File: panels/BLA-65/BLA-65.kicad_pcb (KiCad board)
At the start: 2 copper layers, 60.1 x 128.4 mm, 6 parts

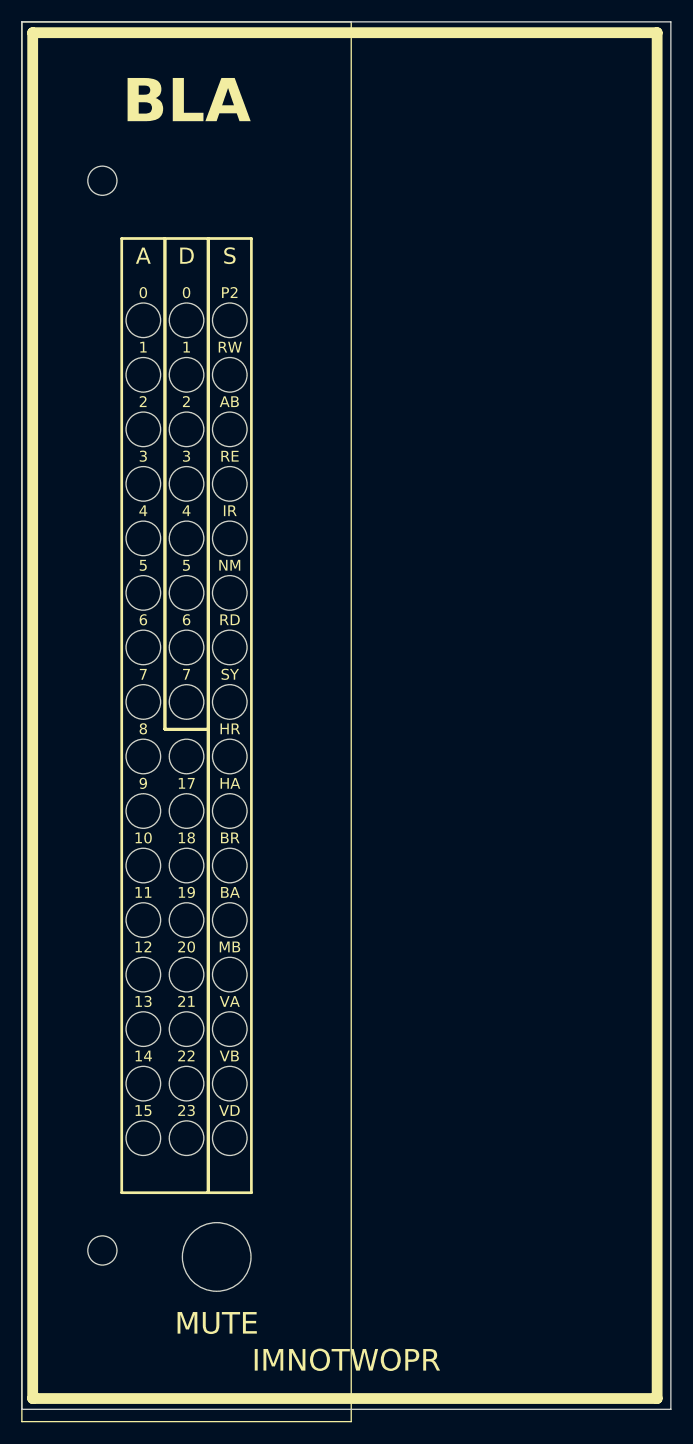
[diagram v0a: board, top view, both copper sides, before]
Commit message: bla panel
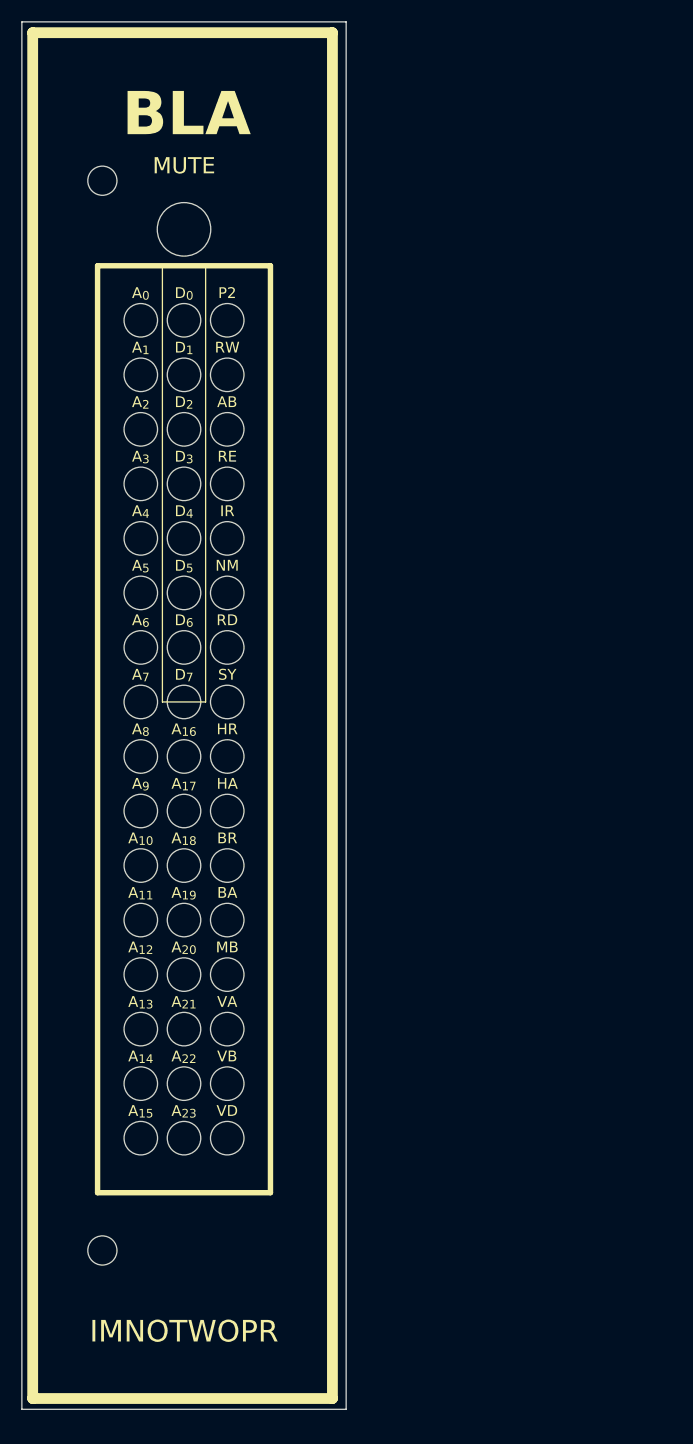
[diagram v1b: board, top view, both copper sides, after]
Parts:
- removed H2: TOP RIGHT, FormantKO-Panel:PanelMountingHole
- removed H4: BOTTOM RIGHT, FormantKO-Panel:PanelMountingHole
- removed the REF** at (84.3, 153.8)
- added REF**: Panel_LED_3.0mm, IMNOTWOPR:Panel_LED_3.0mm, F.Cu at (85.3, 92.4)
- added REF**: Panel_LED_3.0mm, IMNOTWOPR:Panel_LED_3.0mm, F.Cu at (85.3, 137.8)
- added REF**: Panel_LED_3.0mm, IMNOTWOPR:Panel_LED_3.0mm, F.Cu at (77.3, 92.4)
- added REF**: Panel_LED_3.0mm, IMNOTWOPR:Panel_LED_3.0mm, F.Cu at (81.3, 132.7)
- added REF**: Panel_LED_3.0mm, IMNOTWOPR:Panel_LED_3.0mm, F.Cu at (81.3, 72.2)
- added REF**: Panel_LED_3.0mm, IMNOTWOPR:Panel_LED_3.0mm, F.Cu at (85.3, 77.2)
- added REF**: Panel_LED_3.0mm, IMNOTWOPR:Panel_LED_3.0mm, F.Cu at (81.3, 117.6)
- added REF**: Panel_LED_3.0mm, IMNOTWOPR:Panel_LED_3.0mm, F.Cu at (77.3, 132.7)
- added REF**: Panel_LED_3.0mm, IMNOTWOPR:Panel_LED_3.0mm, F.Cu at (81.3, 137.8)
- added REF**: Panel_LED_3.0mm, IMNOTWOPR:Panel_LED_3.0mm, F.Cu at (85.3, 107.5)
- added REF**: Panel_LED_3.0mm, IMNOTWOPR:Panel_LED_3.0mm, F.Cu at (77.3, 102.5)
- added REF**: Panel_LED_3.0mm, IMNOTWOPR:Panel_LED_3.0mm, F.Cu at (81.3, 87.3)
- added REF**: Panel_LED_3.0mm, IMNOTWOPR:Panel_LED_3.0mm, F.Cu at (85.3, 122.6)
- added REF**: Panel_LED_3.0mm, IMNOTWOPR:Panel_LED_3.0mm, F.Cu at (77.3, 72.2)
- added REF**: Panel_LED_3.0mm, IMNOTWOPR:Panel_LED_3.0mm, F.Cu at (85.3, 127.7)
- added REF**: Panel_LED_3.0mm, IMNOTWOPR:Panel_LED_3.0mm, F.Cu at (77.3, 82.3)
- added REF**: Panel_LED_3.0mm, IMNOTWOPR:Panel_LED_3.0mm, F.Cu at (85.3, 132.7)
- added REF**: Panel_LED_3.0mm, IMNOTWOPR:Panel_LED_3.0mm, F.Cu at (77.3, 142.8)
- added REF**: Panel_LED_3.0mm, IMNOTWOPR:Panel_LED_3.0mm, F.Cu at (85.3, 87.3)
- added REF**: Panel_LED_3.0mm, IMNOTWOPR:Panel_LED_3.0mm, F.Cu at (85.3, 67.1)
- added REF**: Panel_LED_3.0mm, IMNOTWOPR:Panel_LED_3.0mm, F.Cu at (85.3, 142.8)
- added REF**: Panel_LED_3.0mm, IMNOTWOPR:Panel_LED_3.0mm, F.Cu at (85.3, 72.2)
- added REF**: Panel_LED_3.0mm, IMNOTWOPR:Panel_LED_3.0mm, F.Cu at (77.3, 77.2)
- added REF**: Panel_LED_3.0mm, IMNOTWOPR:Panel_LED_3.0mm, F.Cu at (81.3, 102.5)
- added REF**: Panel_LED_3.0mm, IMNOTWOPR:Panel_LED_3.0mm, F.Cu at (81.3, 82.3)
- added REF**: Panel_LED_3.0mm, IMNOTWOPR:Panel_LED_3.0mm, F.Cu at (81.3, 92.4)
- added REF**: Panel_LED_3.0mm, IMNOTWOPR:Panel_LED_3.0mm, F.Cu at (85.3, 117.6)
- added REF**: Panel_LED_3.0mm, IMNOTWOPR:Panel_LED_3.0mm, F.Cu at (77.3, 87.3)
- added REF**: Panel_LED_3.0mm, IMNOTWOPR:Panel_LED_3.0mm, F.Cu at (77.3, 67.1)
- added REF**: Panel_LED_3.0mm, IMNOTWOPR:Panel_LED_3.0mm, F.Cu at (85.3, 102.5)
- added REF**: Panel_LED_3.0mm, IMNOTWOPR:Panel_LED_3.0mm, F.Cu at (77.3, 97.4)
- added REF**: Panel_LED_3.0mm, IMNOTWOPR:Panel_LED_3.0mm, F.Cu at (81.3, 112.5)
- added REF**: Panel_LED_3.0mm, IMNOTWOPR:Panel_LED_3.0mm, F.Cu at (85.3, 97.4)
- added REF**: Panel_LED_3.0mm, IMNOTWOPR:Panel_LED_3.0mm, F.Cu at (77.3, 112.5)
- added REF**: Panel_LED_3.0mm, IMNOTWOPR:Panel_LED_3.0mm, F.Cu at (85.3, 82.3)
- added REF**: Panel_LED_3.0mm, IMNOTWOPR:Panel_LED_3.0mm, F.Cu at (77.3, 127.7)
- added REF**: Panel_LED_3.0mm, IMNOTWOPR:Panel_LED_3.0mm, F.Cu at (81.3, 142.8)
- added REF**: Panel_LED_3.0mm, IMNOTWOPR:Panel_LED_3.0mm, F.Cu at (85.3, 112.5)
- added REF**: Panel_LED_3.0mm, IMNOTWOPR:Panel_LED_3.0mm, F.Cu at (77.3, 117.6)
- added REF**: Panel_LED_3.0mm, IMNOTWOPR:Panel_LED_3.0mm, F.Cu at (77.3, 122.6)
- added REF**: Panel_LED_3.0mm, IMNOTWOPR:Panel_LED_3.0mm, F.Cu at (81.3, 127.7)
- added REF**: Panel_LED_3.0mm, IMNOTWOPR:Panel_LED_3.0mm, F.Cu at (81.3, 77.2)
- added REF**: Panel_LED_3.0mm, IMNOTWOPR:Panel_LED_3.0mm, F.Cu at (77.3, 137.8)
- added REF**: Panel_Switch_2M, IMNOTWOPR:Panel_Switch_2M, F.Cu at (81.3, 58.7)
- added REF**: Panel_LED_3.0mm, IMNOTWOPR:Panel_LED_3.0mm, F.Cu at (81.3, 97.4)
- added REF**: Panel_LED_3.0mm, IMNOTWOPR:Panel_LED_3.0mm, F.Cu at (81.3, 67.1)
- added REF**: Panel_LED_3.0mm, IMNOTWOPR:Panel_LED_3.0mm, F.Cu at (77.3, 107.5)
- added REF**: Panel_LED_3.0mm, IMNOTWOPR:Panel_LED_3.0mm, F.Cu at (81.3, 122.6)
- added REF**: Panel_LED_3.0mm, IMNOTWOPR:Panel_LED_3.0mm, F.Cu at (81.3, 107.5)
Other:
- board size 60.1 x 128.4 mm -> 30 x 128.4 mm
- board text added: "A_{0}"
- board text added: "A_{10}"
- board text added: "A_{11}"
- board text added: "A_{12}"
- board text added: "A_{13}"
- board text added: "A_{14}"
- board text added: "A_{15}"
- board text added: "A_{16}"
- board text added: "A_{17}"
- board text added: "A_{18}"
- board text added: "A_{19}"
- board text added: "A_{1}"
- board text added: "A_{20}"
- board text added: "A_{21}"
- board text added: "A_{22}"
- board text added: "A_{23}"
- board text added: "A_{2}"
- board text added: "A_{3}"
- board text added: "A_{4}"
- board text added: "A_{5}"
- board text added: "A_{6}"
- board text added: "A_{7}"
- board text added: "A_{8}"
- board text added: "A_{9}"
- board text added: "D_{0}"
- board text added: "D_{1}"
- board text added: "D_{2}"
- board text added: "D_{3}"
- board text added: "D_{4}"
- board text added: "D_{5}"
- board text added: "D_{6}"
- board text added: "D_{7}"
- board text removed: "0"
- board text removed: "1"
- board text removed: "10"
- board text removed: "11"
- board text removed: "12"
- board text removed: "13"
- board text removed: "14"
- board text removed: "15"
- board text removed: "17"
- board text removed: "18"
- board text removed: "19"
- board text removed: "2"
- board text removed: "20"
- board text removed: "21"
- board text removed: "22"
- board text removed: "23"
- board text removed: "3"
- board text removed: "4"
- board text removed: "5"
- board text removed: "6"
- board text removed: "7"
- board text removed: "8"
- board text removed: "9"
- board text removed: "A"
- board text removed: "D"
- board text removed: "S"
